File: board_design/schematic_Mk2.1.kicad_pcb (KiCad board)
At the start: 2 copper layers, 82.8 x 74 mm, 32 parts, among them J1 A-DF_09_A_KG-T4S, J2 1757255, J3 JST -SM, J4 S3B-EH, U1 ESP32-DEVKITC-32D, U2 LTV-846S

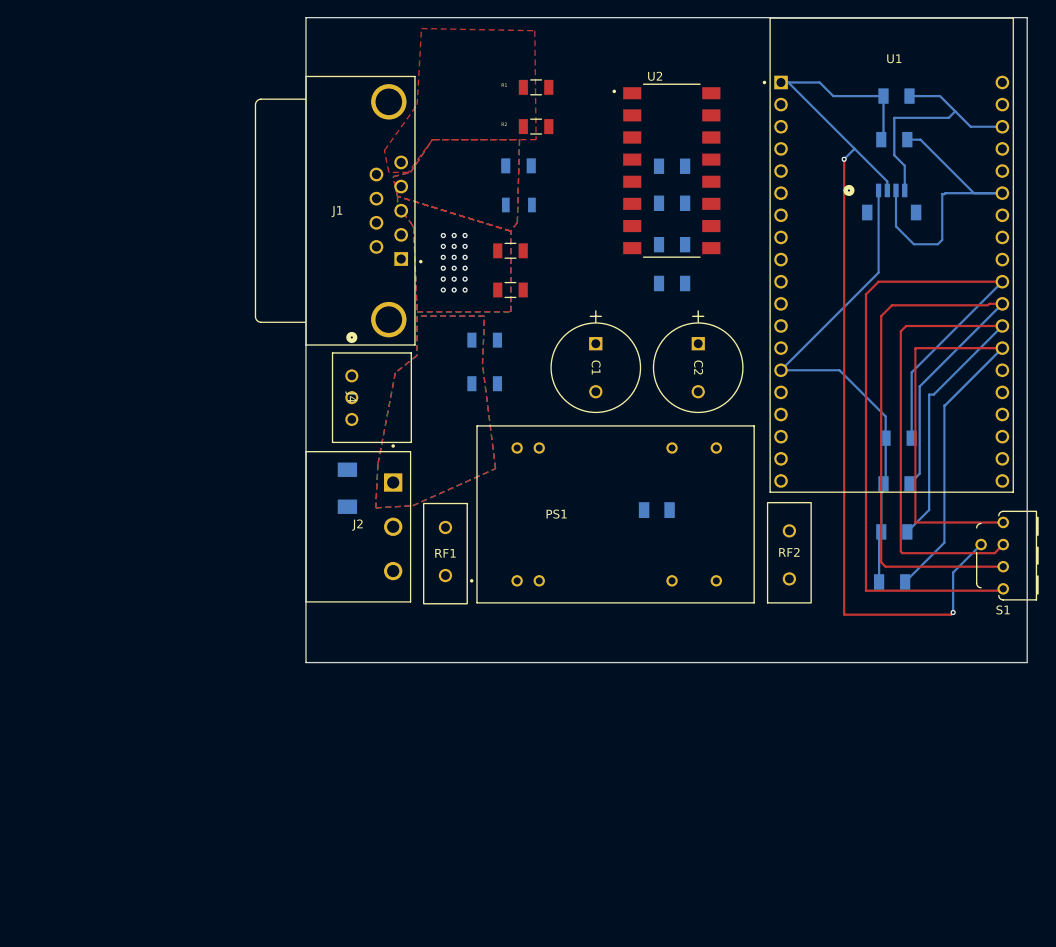
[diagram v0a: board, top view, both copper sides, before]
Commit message: update
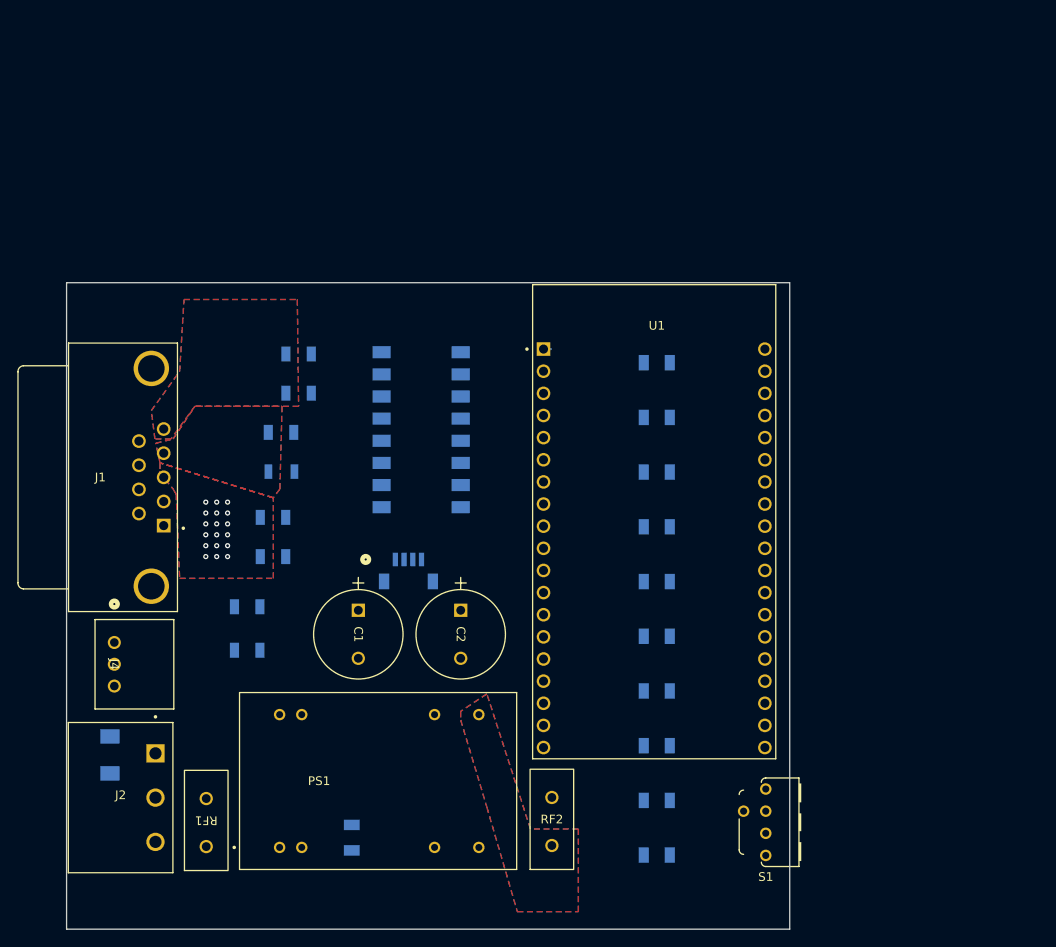
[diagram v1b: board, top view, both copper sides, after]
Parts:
- R1, R2, R5, R6, U2: moved to B.Cu
- moved J3 69.8 mm to (134.8, 88.6)
- moved C3 51.4 mm to (128.2, 119.1), turned to -90 degrees
- moved RF1 45.8 mm to (111.5, 120.1), turned to 90 degrees
- moved R17 41.9 mm to (163.2, 70.9)
- moved R16 41.4 mm to (163.2, 121.1)
- moved U2 41.4 mm to (136.2, 72.3)
- moved J2 41.3 mm to (95.7, 105.9)
- moved R18 41.1 mm to (163.2, 64.6)
- moved R15 41.1 mm to (163.2, 114.8)
- moved R5 41.0 mm to (119.2, 82.3)
- moved R6 41.0 mm to (119.2, 86.8)
- moved D1 41.0 mm to (100.5, 109.6)
- moved PS1 41.0 mm to (131.3, 112.6)
- moved R2 41.0 mm to (122.2, 68.1)
- moved R3 41.0 mm to (120.1, 72.6)
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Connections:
- C3 pad 1: -VOUT -> ESP_GND2
- PS1 pad 16: -VOUT -> ESP_GND2
- U1 pad J3-1: -VOUT -> ESP_GND2
- U2 pad 1: Net-(R1-Pad2) -> Net-(R7-Pad2)
- U2 pad 10: GPIO_26 -> GPIO_32
- U2 pad 12: GPIO_25 -> GPIO_33
- U2 pad 14: GPIO_33 -> GPIO_25
- U2 pad 16: GPIO_32 -> GPIO_26
- U2 pad 3: Net-(R3-Pad2) -> Net-(R5-Pad2)
- U2 pad 5: Net-(R5-Pad2) -> Net-(R3-Pad2)
- U2 pad 7: Net-(R7-Pad2) -> Net-(R1-Pad2)
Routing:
- net +3.3V: track 111.1 -> 0.84 mm, vias 2 -> 0
- net GPIO_5: track 88.3 -> 0.30 mm
- net GPIO_17: track 82.0 -> 0.00 mm
- net GPIO_16: track 77.8 -> 0.00 mm
- net GPIO_4: track 71.6 -> 0.00 mm
- net ESP_GND2: track 58.8 -> 0.00 mm
- net GPIO_21: track 36.1 -> 0.00 mm
- net GPIO_22: track 29.0 -> 0.00 mm
- added copper zone on B.Cu, net +VOUT
- added copper zone on F.Cu, net +VOUT
- added copper zone on B.Cu, net spare
- removed copper zone on B.Cu, net sim_home
- removed copper zone on F.Cu, net sim_home
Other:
- board size 82.8 x 74 mm -> 83 x 74.2 mm
